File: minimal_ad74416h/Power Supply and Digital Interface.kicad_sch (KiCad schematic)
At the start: 62 parts, among them T1 ZA9644-AED, U4 MAX17570FATA+, U5 MAX17614ATP+, U6 ADP1031ACPZ-3-R7, U7 ADUM1252AUA+

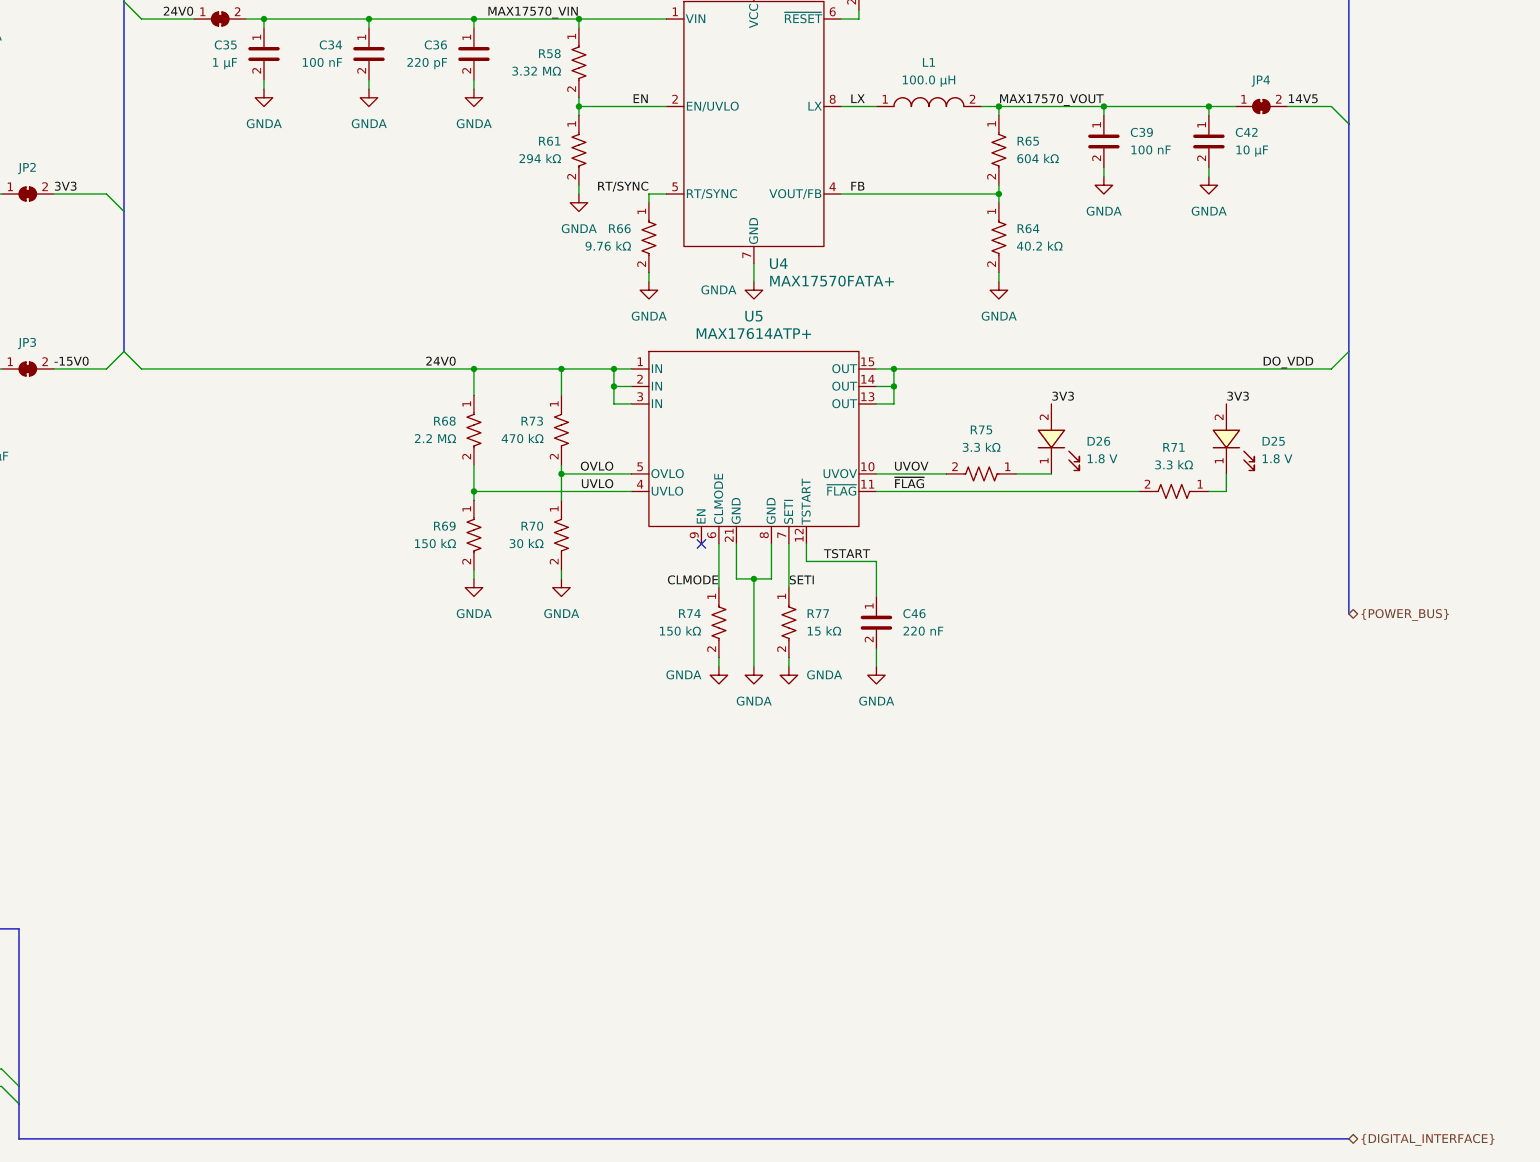
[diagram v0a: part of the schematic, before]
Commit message: backup
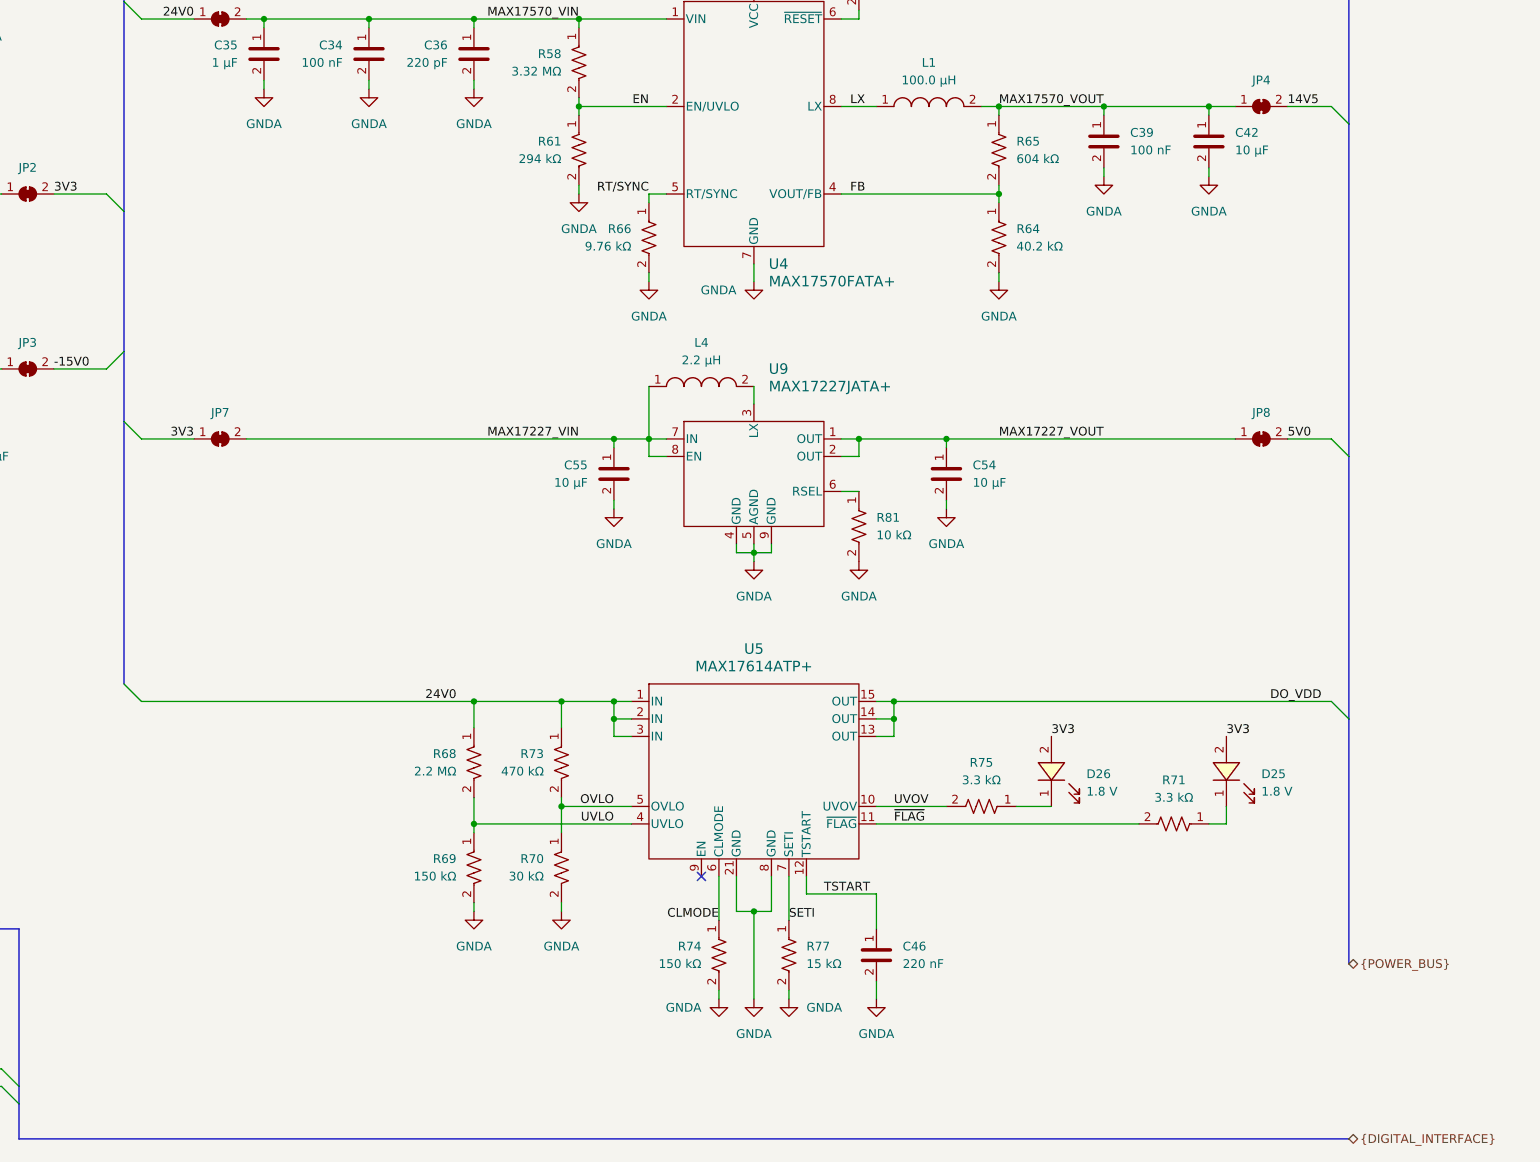
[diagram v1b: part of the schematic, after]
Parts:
- added C54, C55: 10 µF, capacitor_footprints:C_0603_1608Metric, symbol CAPACITORS_C1608X5R1C_DATA_BASE:C_C1608X5R1C106M080AB
- added JP7, JP8: SolderJumper_2_Bridged, solder_jumper_footprints:SolderJumper-2_P1.3mm_Bridged_RoundedPad1.0x1.5mm, symbol UNITED_SOLDER_JUMPERS:SolderJumper_2_Bridged
- added L4: 2.2 µH, inductor_footprints:74479276, symbol UNITED_INDUCTORS_DATA_BASE:L_74479276222
- added R81: 10 kΩ, resistor_footprints:R_0402_1005Metric, symbol UNITED_RESISTORS_DATA_BASE:R_ERJ-2RKF1002X
- added U9: MAX17227JATA+, analog_devices_footprints:21-0168_T822&plus_3C_ADI, symbol UNITED_IC_ADI:U_MAX17227JATA+
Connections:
- net 3V3: now also JP7.1
- net GNDA: now also C54.2, C55.2, R81.2, U9.4 (GND), U9.5 (AGND), U9.9 (GND)
- new net: R81.1, U9.6 (RSEL)
- new net: L4.2, U9.3 (LX)
- new net 5V0: JP8.2
- new net MAX17227_VIN: C55.1, JP7.2, L4.1, U9.7 (IN), U9.8 (EN)
- new net MAX17227_VOUT: C54.1, JP8.1, U9.1 (OUT), U9.2 (OUT)
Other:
- moved on the sheet: C46, D25, D26, R68, R69, R70, R71, R73, R74, R75, R77, U5
